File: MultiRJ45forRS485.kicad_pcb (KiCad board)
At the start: 2 copper layers, 100 x 100 mm, 1 part, among them X1 RJ45_56LED_2*2_1

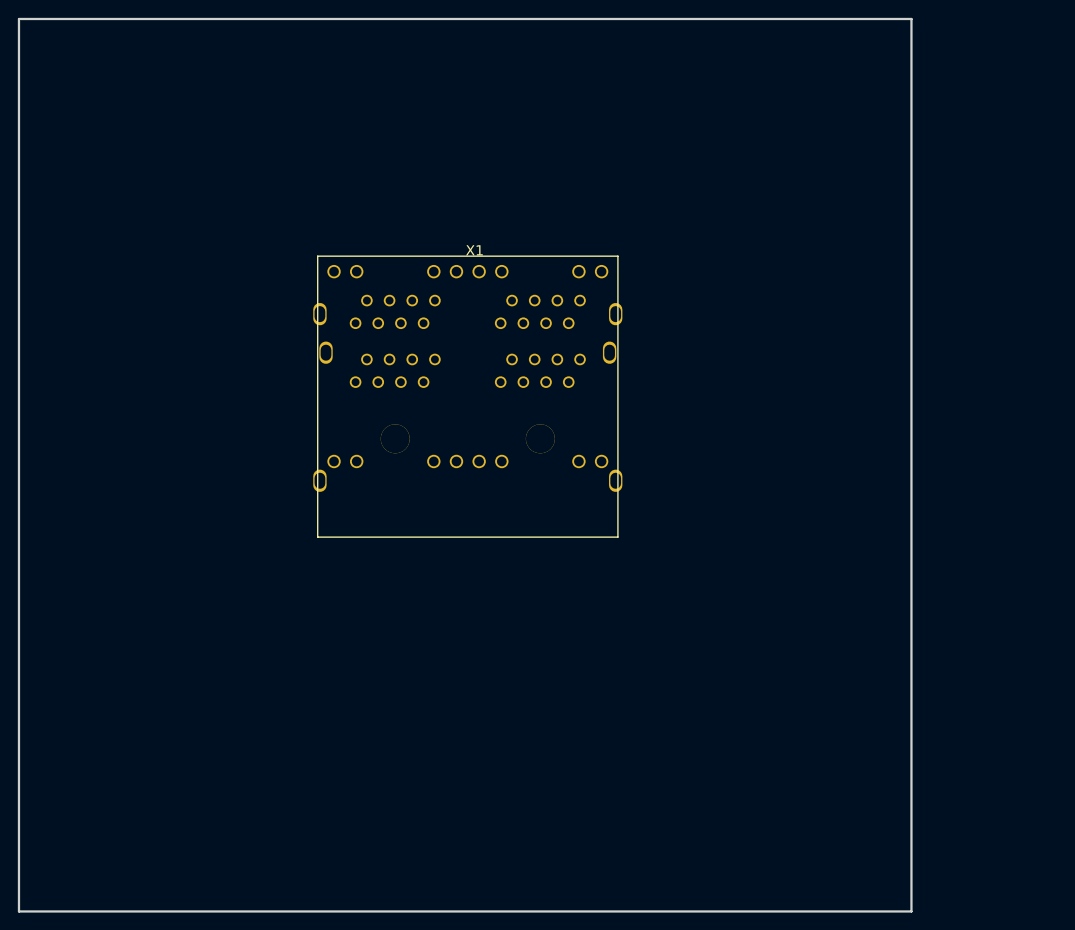
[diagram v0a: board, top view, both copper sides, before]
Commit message: Create PCB
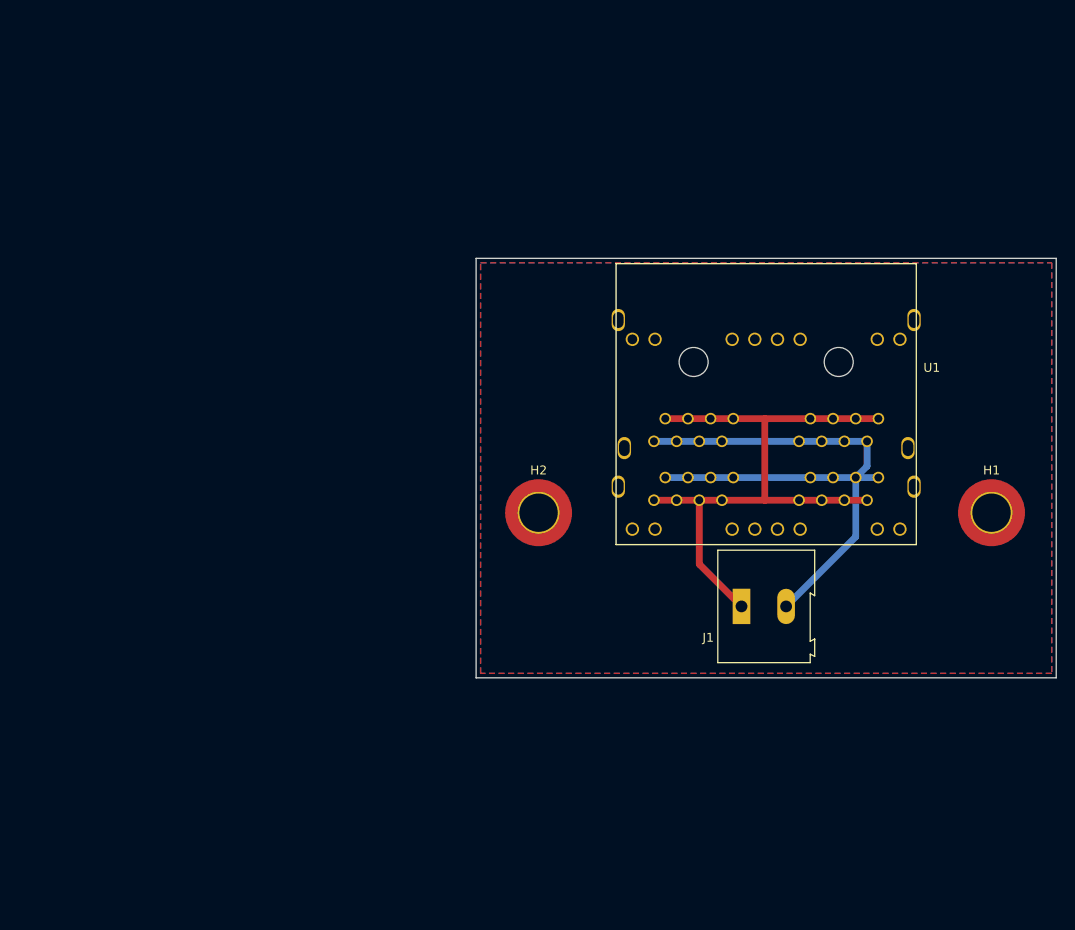
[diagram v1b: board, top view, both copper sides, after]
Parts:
- removed X1: RJ45_56LED_2*2_1, easyeda:RJ45_56LED_2*2_1
- added H1: MountingHole_Pad, MountingHole:MountingHole_4.3mm_M4_DIN965_Pad_TopOnly, F.Cu at (126.8, 54.0)
- added H2: MountingHole_Pad, MountingHole:MountingHole_4.3mm_M4_DIN965_Pad_TopOnly, F.Cu at (76.0, 54.0)
- added J1: Screw_Terminal_01x02, TerminalBlock:TerminalBlock_Altech_AK300-2_P5.00mm, F.Cu at (98.7, 64.5)
- added U1: RJ45_56LED_2*2, PcbLib:RJ45_56LED_2*2, F.Cu at (100.4, 42.7)
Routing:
- net Net-(J1-Pad1): track 0.00 -> 70.8 mm
- net Net-(J1-Pad2): track 0.00 -> 70.0 mm
- added copper zone on B.Cu, net Net-(H1-Pad1)
- added copper zone on F.Cu, net Net-(H1-Pad1)
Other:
- board size 100 x 100 mm -> 65 x 47 mm
